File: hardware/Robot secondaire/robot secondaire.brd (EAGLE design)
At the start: 85.1 x 39 mm, 27 parts, among them IC1 7812TV

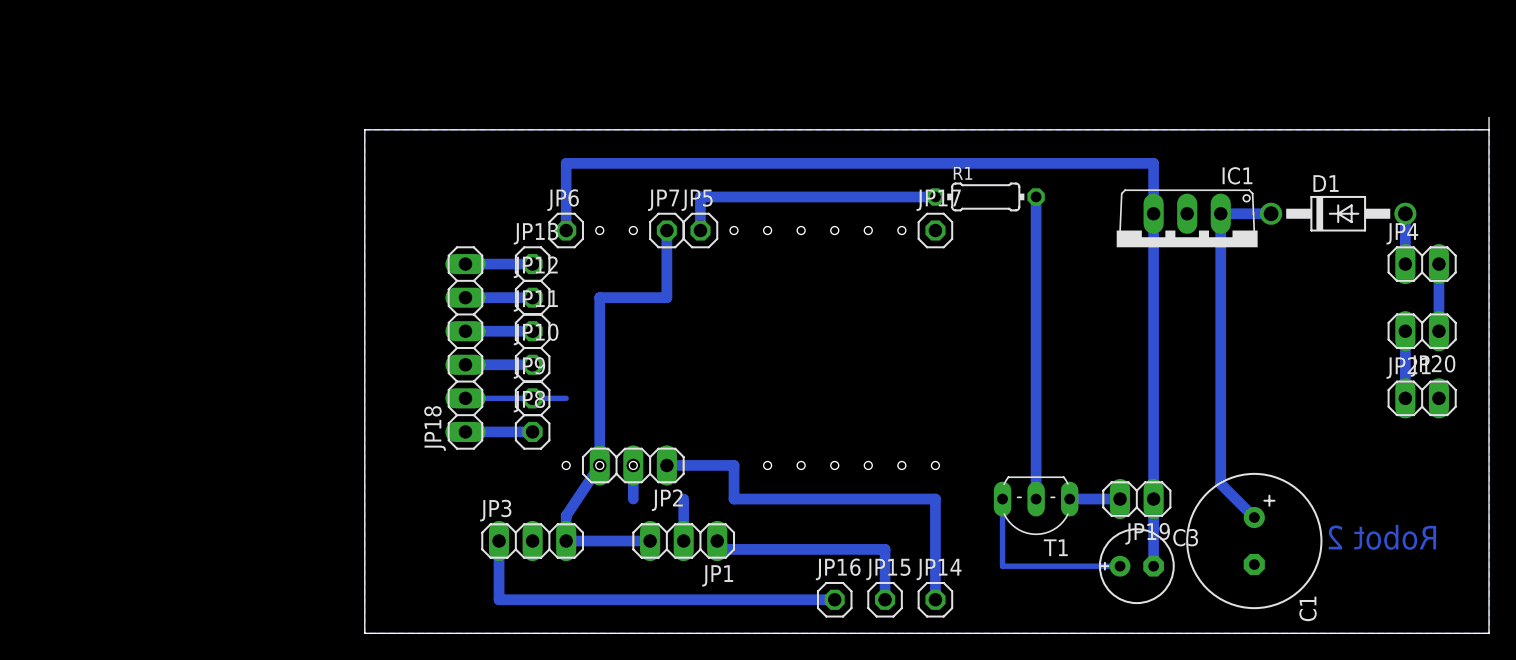
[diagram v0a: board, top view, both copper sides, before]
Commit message: maj elec robot secondaire
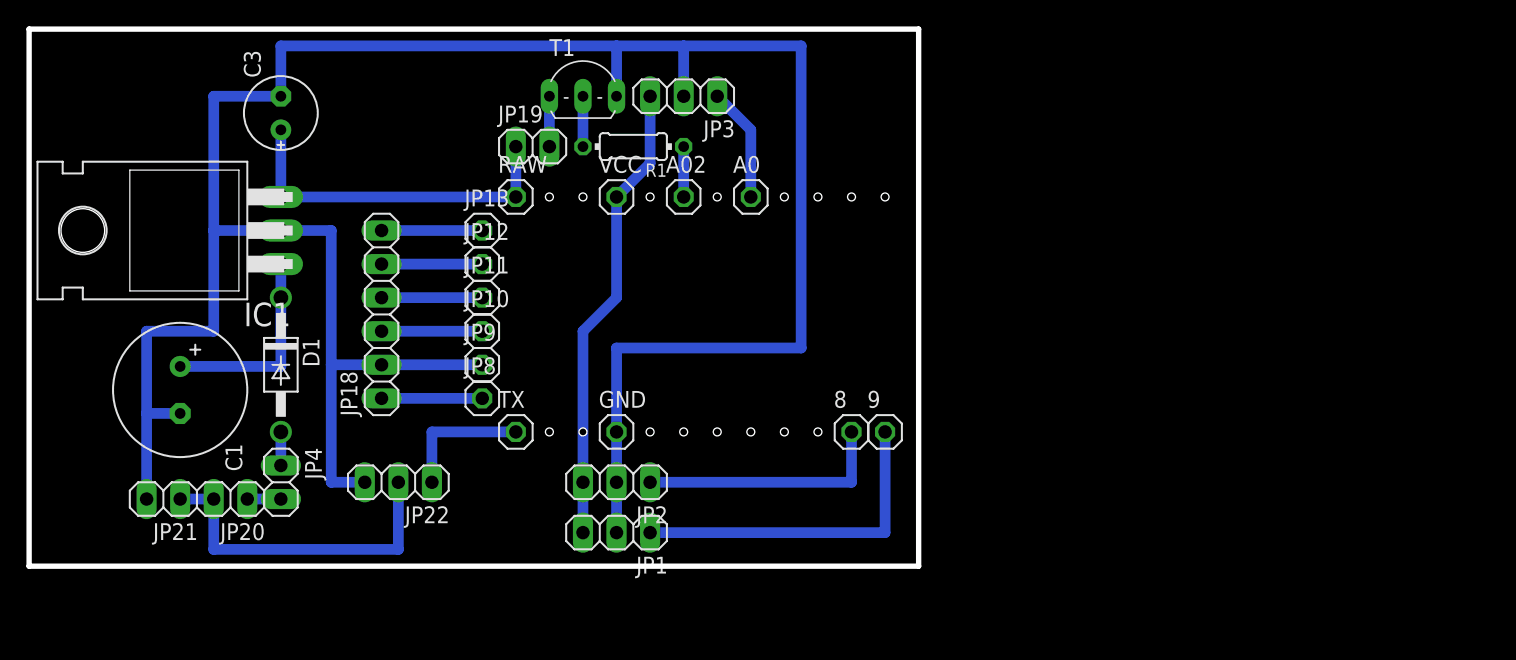
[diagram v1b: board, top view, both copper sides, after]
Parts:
- removed JP14, JP15, JP16, JP17, JP5, JP6, JP7: (no value), pinhead:1X01
- added 8, 9, A0, A02, GND, RAW, TX, VCC: (no value), pinhead:1X01
- added JP22: (no value), pinhead:1X03
- IC1: value 7812TV -> 7812T; device linear:TO220V -> linear:TO220H
- moved JP21 95.6 mm to (-19.1, 73.7), turned to 180 degrees
- moved JP20 91.1 mm to (-14.0, 73.7)
- moved JP4 87.9 mm to (-10.2, 74.9), turned to 270 degrees
- moved C1 82.1 mm to (-17.8, 81.9)
- moved D1 80.8 mm to (-10.2, 83.8), turned to 270 degrees
- moved IC1 78.8 mm to (-20.3, 94.0), turned to 90 degrees
- moved C3 73.3 mm to (-10.2, 102.9), turned to 90 degrees
- moved JP19 52.9 mm to (8.89, 100.3), turned to 0 degrees
- moved T1 45.9 mm to (12.7, 104.1), turned to 0 degrees
- moved JP3 35.5 mm to (20.3, 104.1), turned to 180 degrees
- moved R1 26.9 mm to (16.5, 100.3), turned to 180 degrees
- moved JP18 6.84 mm to (-2.54, 87.6)
- moved JP1 5.12 mm to (15.2, 71.1)
- moved JP10 4.58 mm to (5.08, 86.4)
- moved JP11 4.58 mm to (5.08, 88.9)
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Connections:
- removed net N$10: JP20.2, JP21.1
- removed net N$9: JP5.1, R1.1
- new net +9V: JP20.2, JP21.1, JP22.2
- new net AX12: JP22.1, TX.1
- new net CMD_MOTEUR: A02.1, R1.1
- net +12V: now also C3.+, RAW.1; no longer C3.-, JP6.1
- net +5V: now also VCC.1; no longer JP7.1
- net C: now also 9.1; no longer JP15.1
- net DAC: now also A0.1; no longer JP16.1
- net GND: now also C3.-, GND.1, JP22.3; no longer C3.+, JP17.1
- net J: now also 8.1; no longer JP14.1
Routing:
- net GND: track 29.2 -> 186.7 mm
- net +12V: track 80.0 -> 26.7 mm
- net +9V: track 0.00 -> 25.4 mm
- net DAC: track 29.8 -> 8.67 mm
- net N$9: track 20.3 -> 0.00 mm
- net N$6: track 22.9 -> 3.81 mm
- net N$1: track 27.8 -> 15.4 mm
- net J: track 30.5 -> 19.0 mm
- net AX12: track 0.00 -> 10.2 mm
- net C: track 16.8 -> 25.4 mm
- net N$10: track 5.08 -> 0.00 mm
- net CMD_MOTEUR: track 0.00 -> 3.81 mm
- net VCC: track 5.08 -> 7.62 mm
- net TXI: track 5.08 -> 7.62 mm
- net RXI: track 5.08 -> 7.62 mm
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- removed copper zone on layer 16, net GND
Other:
- board size 85.1 x 39 mm -> 67.3 x 40.6 mm
- board text removed: "Robot 2"
